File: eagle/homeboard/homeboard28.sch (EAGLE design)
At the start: 126 parts, among them IC1 XCF02S, IC2 25LC080SN, IC3 ATMEGA32U2-TQFP, Q5 BC848SMD, Q6 BC848SMD, Q7 BC848SMD, Q8 BC848SMD, T1 BSS138, T2 BC848, T3 BSS138, U1 XC3S400TQ144, X1 SCART-CLIP, X6 MINI-USB_4P-85-32004-10X, X7 DC21MMX, X8 STEREOJACK

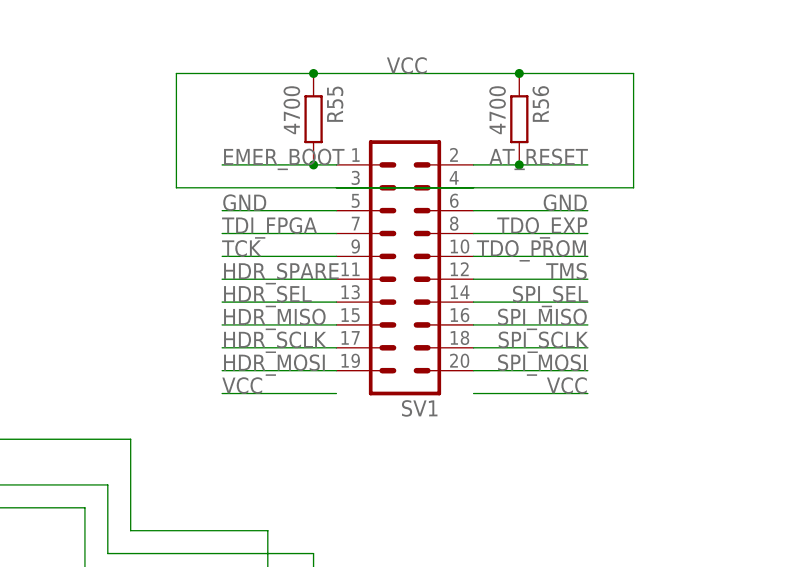
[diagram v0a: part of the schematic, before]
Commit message: maybe final
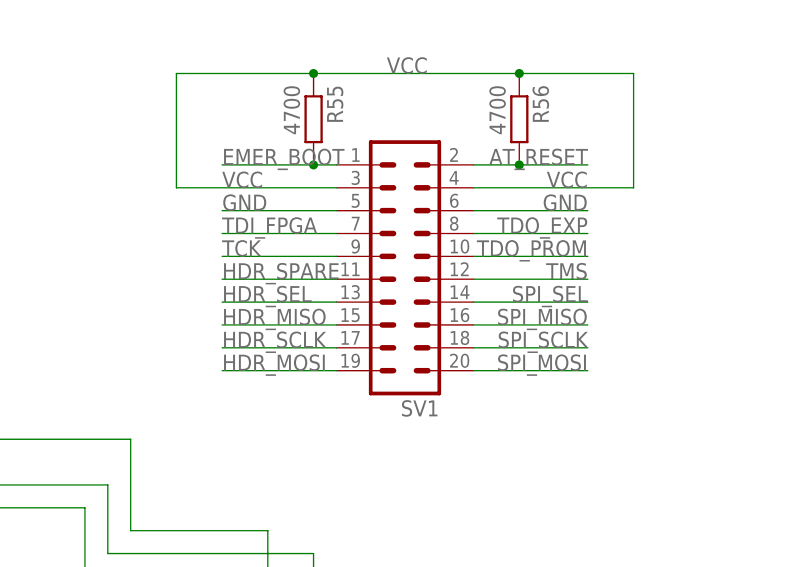
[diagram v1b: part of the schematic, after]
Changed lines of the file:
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@@
 </segment>
 <segment>
+<wire x1="327.66" y1="40.64" x2="309.88" y2="40.64" width="0.1524" layer="91"/>
+<label x="322.58" y="40.64" size="1.778" layer="95" rot="MR0"/>
+<wire x1="276.86" y1="40.64" x2="294.64" y2="40.64" width="0.1524" layer="91"/>
+<label x="281.94" y="40.64" size="1.778" layer="95"/>
 <pinref part="R55" gate="G$1" pin="1"/>
 <pinref part="R56" gate="G$1" pin="1"/>
 <wire x1="292.1" y1="53.34" x2="314.96" y2="53.34" width="0.1524" layer="91"/>
 <label x="304.8" y="53.34" size="1.778" layer="95" rot="MR0"/>
-<pinref part="SV1" gate="G$1" pin="3"/>
-<wire x1="294.64" y1="40.64" x2="327.66" y2="40.64" width="0.1524" layer="91"/>
 <wire x1="327.66" y1="40.64" x2="327.66" y2="53.34" width="0.1524" layer="91"/>
 <wire x1="327.66" y1="53.34" x2="314.96" y2="53.34" width="0.1524" layer="91"/>
 <junction x="314.96" y="53.34"/>
-<pinref part="SV1" gate="G$1" pin="4"/>
-<wire x1="309.88" y1="40.64" x2="276.86" y2="40.64" width="0.1524" layer="91"/>
 <wire x1="276.86" y1="40.64" x2="276.86" y2="53.34" width="0.1524" layer="91"/>
 <wire x1="276.86" y1="53.34" x2="292.1" y2="53.34" width="0.1524" layer="91"/>
 <junction x="292.1" y="53.34"/>
+<pinref part="SV1" gate="G$1" pin="3"/>
+<pinref part="SV1" gate="G$1" pin="4"/>
 </segment>
 <segment>
-<wire x1="281.94" y1="17.78" x2="294.64" y2="17.78" width="0.1524" layer="91"/>
-<label x="281.94" y="17.78" size="1.778" layer="95"/>
-</segment>
-<segment>
-<wire x1="322.58" y1="17.78" x2="309.88" y2="17.78" width="0.1524" layer="91"/>
-<label x="322.58" y="17.78" size="1.778" layer="95" rot="MR0"/>
-</segment>
-<segment>
